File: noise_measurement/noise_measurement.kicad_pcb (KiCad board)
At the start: 2 copper layers, 15 x 19.4 mm, 16 parts, among them U1 OPA344, U2 MSP430G2210ID, U3 SPH8878LR5H-2

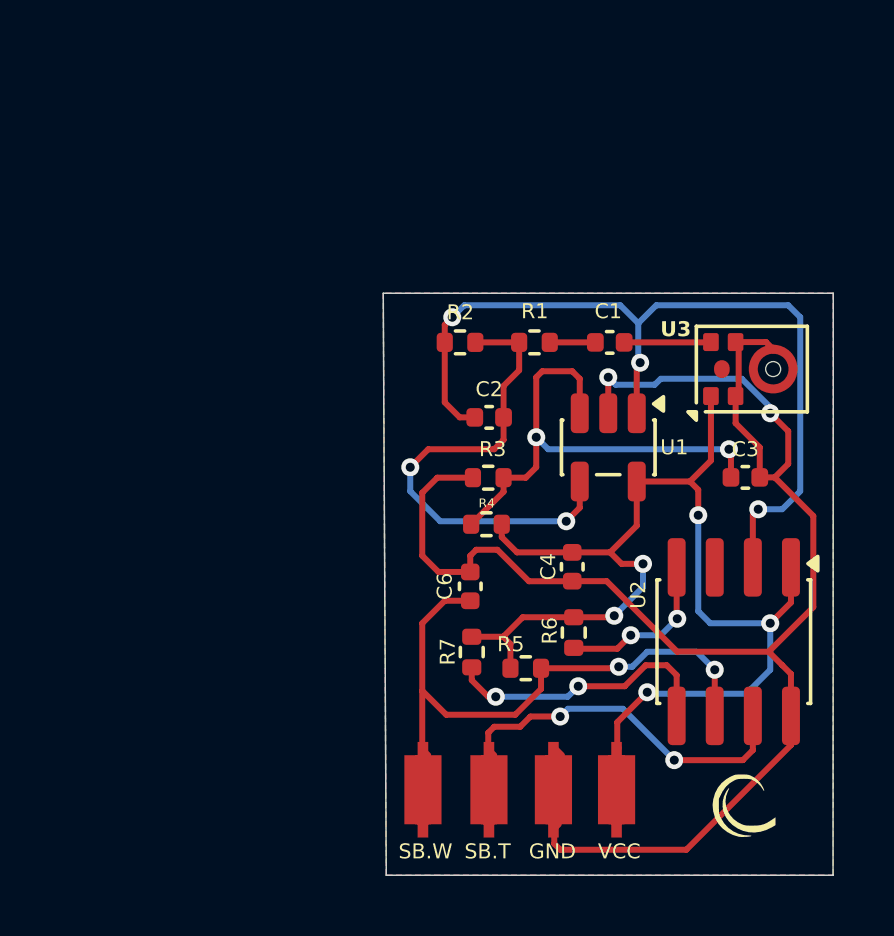
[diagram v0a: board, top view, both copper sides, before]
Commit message: Add files via upload
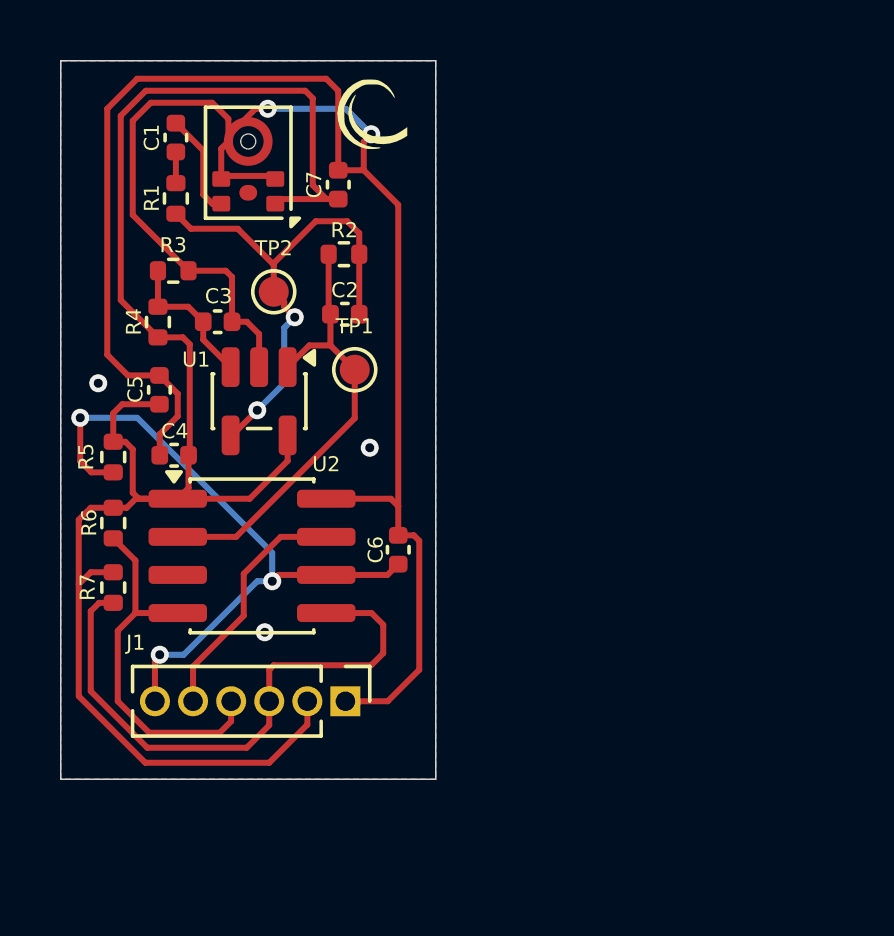
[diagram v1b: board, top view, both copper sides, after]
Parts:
- added C5: 0.1uF, Capacitor_SMD:C_0402_1005Metric, F.Cu at (83.0, 43.8)
- added C7: 0.1uF, Capacitor_SMD:C_0402_1005Metric, F.Cu at (89.0, 37.0)
- added J1: Conn_01x06_Pin, Connector_PinHeader_1.27mm:PinHeader_1x06_P1.27mm_Vertical, F.Cu at (89.2, 54.2)
- added TP1: TestPoint, TestPoint:TestPoint_Pad_D1.0mm, F.Cu at (89.5, 43.1)
- added TP2: TestPoint, TestPoint:TestPoint_Pad_D1.0mm, F.Cu at (86.8, 40.5)
- moved G*** 26.2 mm to (90.0, 34.6)
- moved U3 20.1 mm to (87.6, 34.2), turned to 180 degrees
- moved C3 18.3 mm to (85.0, 41.5)
- moved U2 16.3 mm to (86.1, 49.4), turned to 0 degrees
- moved C1 16.0 mm to (83.6, 35.4), turned to 90 degrees
- moved R6 15.8 mm to (81.5, 48.3)
- moved R5 15.4 mm to (81.5, 46.1), turned to 90 degrees
- moved C4 13.8 mm to (83.5, 46.0), turned to 0 degrees
- moved R1 12.9 mm to (83.6, 37.4), turned to 90 degrees
- moved R4 12.9 mm to (83.0, 41.6), turned to 90 degrees
- moved R3 12.6 mm to (83.5, 39.9), turned to 0 degrees
- moved R7 12.1 mm to (81.5, 50.4)
- moved U1 11.7 mm to (86.4, 44.2)
- moved C2 5.91 mm to (89.2, 41.3)
- moved R2 4.86 mm to (89.2, 39.3)
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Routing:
- net VCC: track 38.9 -> 58.3 mm, vias 5 -> 0
- net GND: track 55.7 -> 73.9 mm, vias 2 -> 5
- net Net-(U2-TA0.1/CA2/P1.2): track 29.1 -> 15.1 mm, vias 3 -> 0
- net Net-(U1-+): track 16.6 -> 4.81 mm, vias 2 -> 0
- net /SDA: track 9.42 -> 19.5 mm, vias 2 -> 0
- net /SCL: track 5.60 -> 12.4 mm, vias 2 -> 0
- net /SBTCK: track 12.0 -> 8.21 mm, vias 2 -> 0
- net /SBWTDIO: track 19.6 -> 22.7 mm, vias 2 -> 3
- net Net-(U1--): track 16.3 -> 17.2 mm
- net Net-(U3-OUT(+)): track 2.90 -> 3.49 mm
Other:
- board size 15 x 19.4 mm -> 12.5 x 23.9 mm
- board text removed: "GND"
- board text removed: "SB.T"
- board text removed: "SB.W"
- board text removed: "VCC"
